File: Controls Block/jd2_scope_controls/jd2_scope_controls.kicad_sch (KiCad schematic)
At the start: 20 parts, among them SW1 RotaryEncoder_Switch, SW2 RotaryEncoder_Switch, SW3 RotaryEncoder_Switch, SW4 SW_SPST

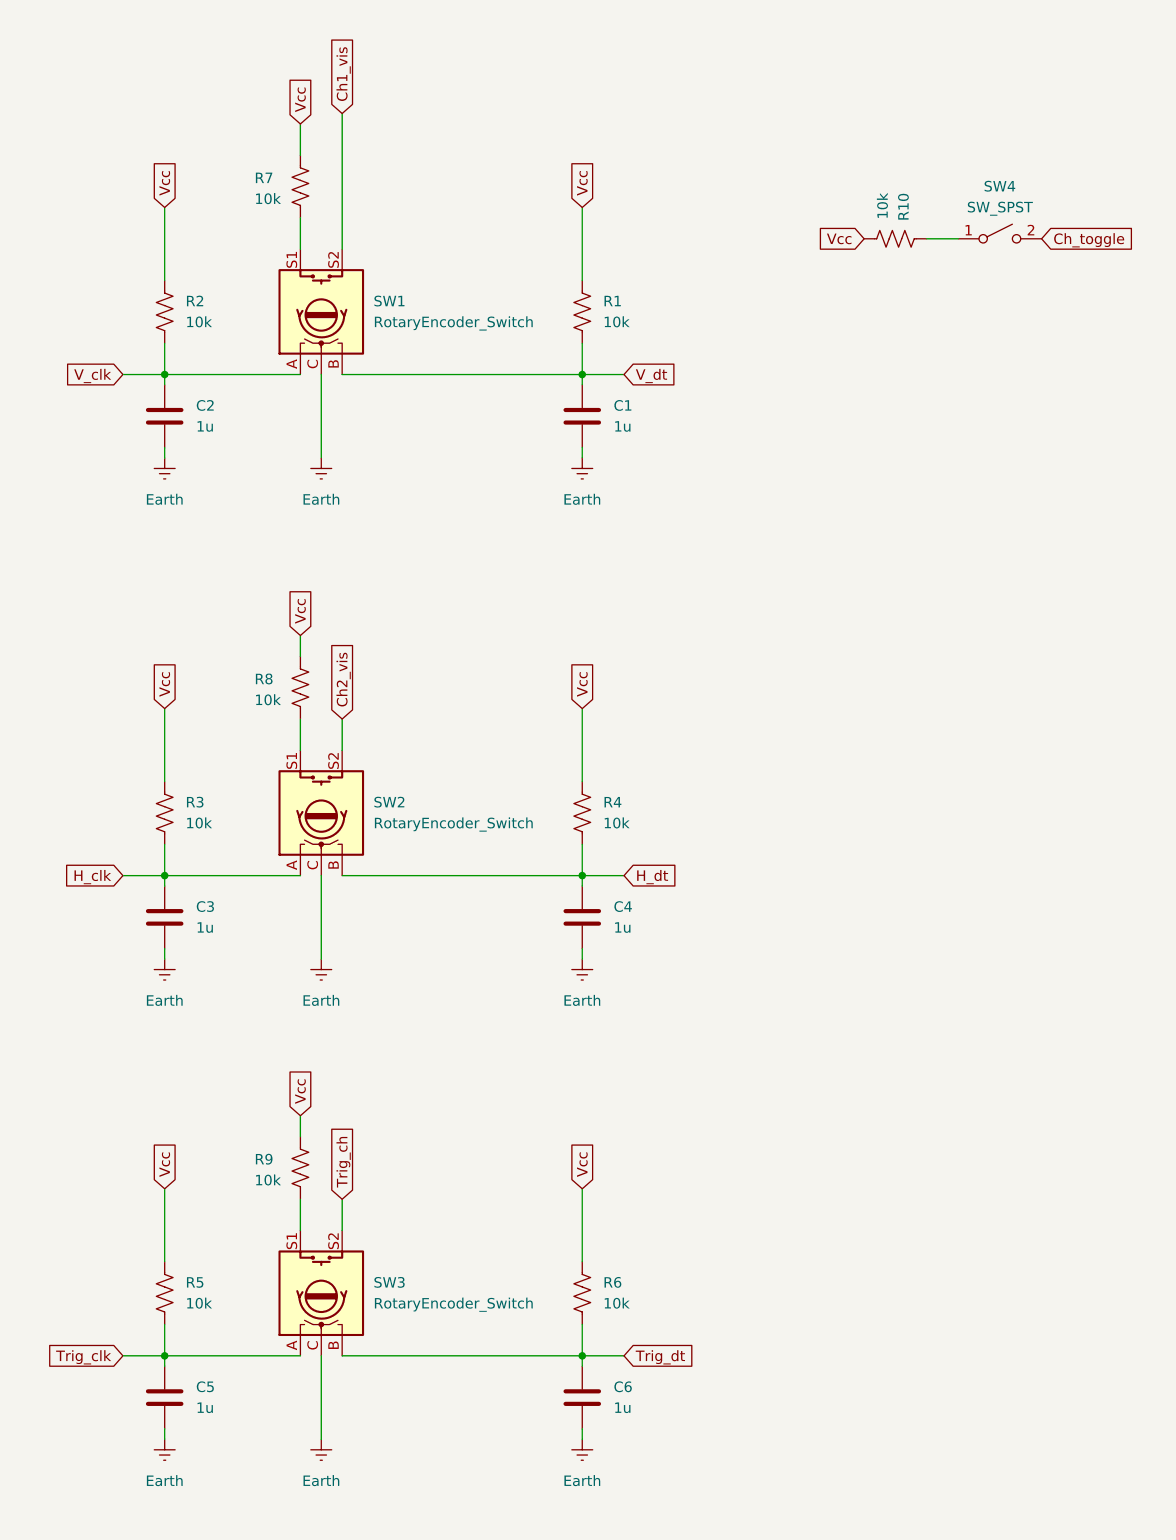
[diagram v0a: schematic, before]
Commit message: footprint stuff
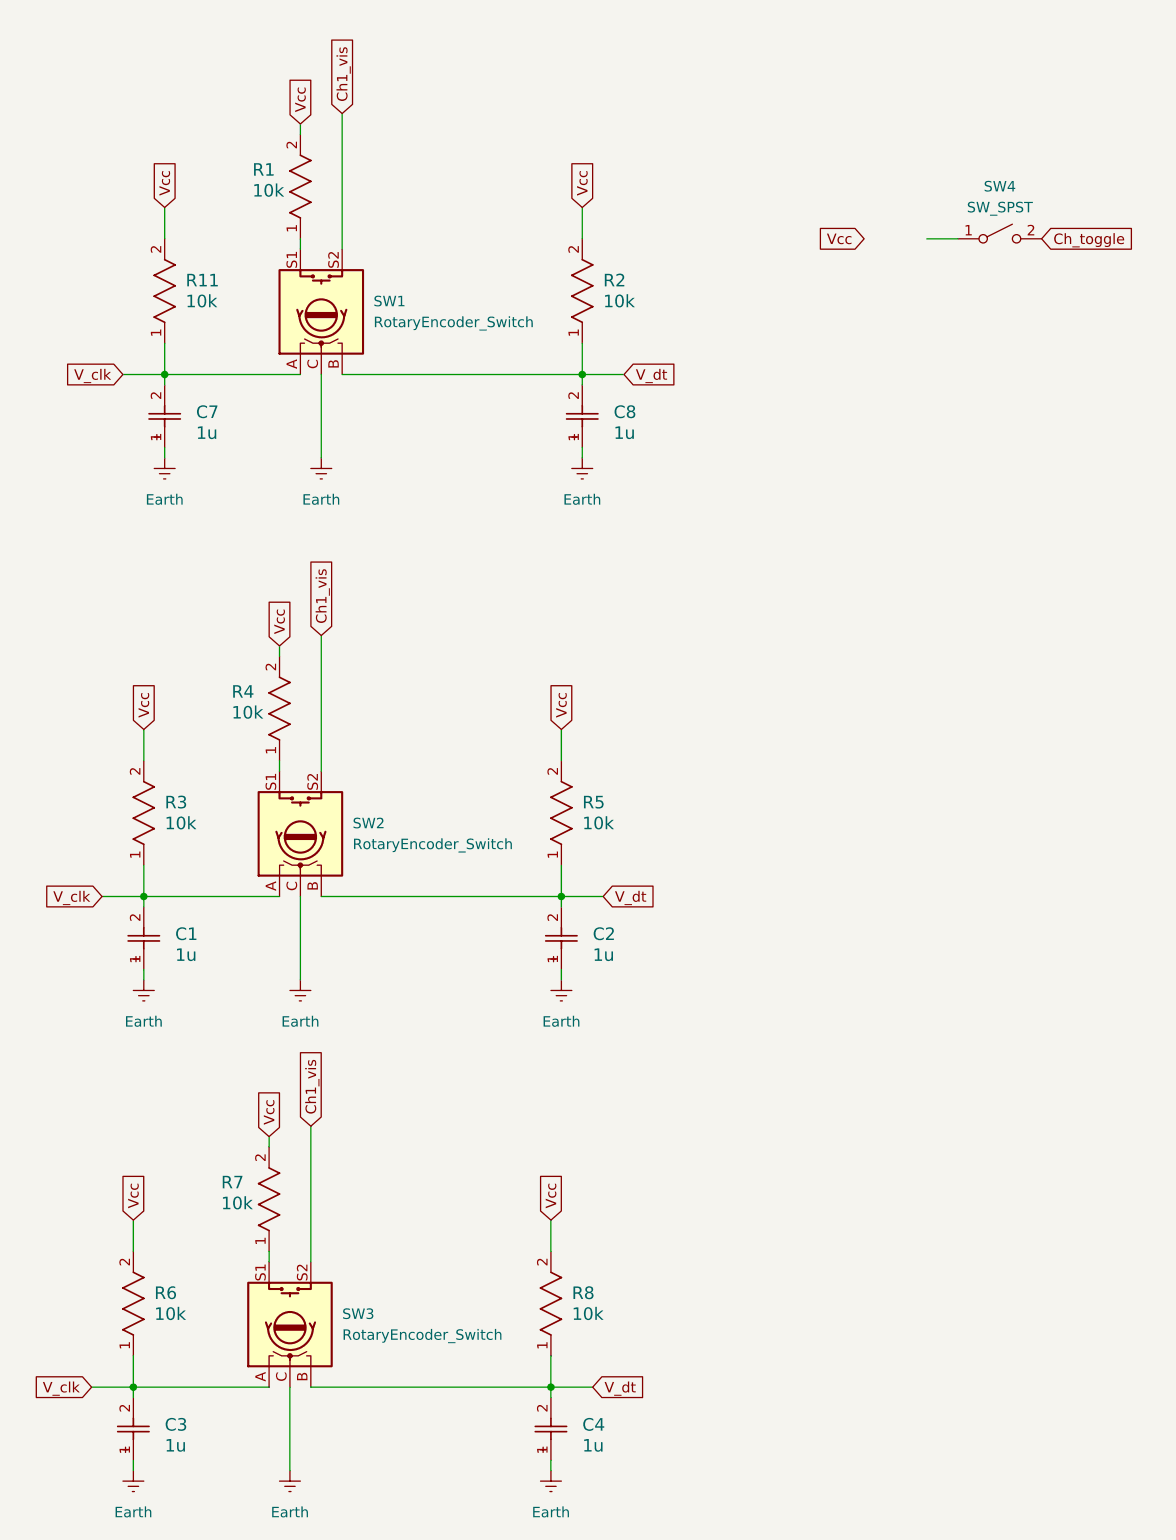
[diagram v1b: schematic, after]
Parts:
- removed C1, C2, C3, C4, C5, C6: 1u, symbol Device:C
- removed R1, R10, R2, R3, R4, R5, R6, R7, R8, R9: 10k, symbol Device:R_US
- added C1, C2, C3, C4, C7, C8: 1u, CAP_UEP_6P3X11_NCH, symbol fp1:UVZ2F010MED1TD
- added R1, R11, R2, R3, R4, R5, R6, R7, R8: 10k, STA_RMCF0402_STP, symbol fp1:RMCF0402FT10K0
- SW4: footprint (none) -> Button_Switch_SMD:Nidec_Copal_CAS-120A
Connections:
- net Ch2_vis is gone; now on net Ch1_vis: SW2.S2
- net H_clk is gone; now on net V_clk: SW2.A
- net H_dt is gone; now on net V_dt: SW2.B
- net Trig_ch is gone; now on net Ch1_vis: SW3.S2
- net Trig_clk is gone; now on net V_clk: SW3.A
- net Trig_dt is gone; now on net V_dt: SW3.B
- net Earth: now also C1.1, C2.1, C3.1, C4.1, C7.1, C8.1
- net V_clk: now also C1.2, C3.2, C7.2, R11.1, R3.1, R6.1
- net V_dt: now also C2.2, C4.2, C8.2, R2.1, R5.1, R8.1
- net Vcc: now also R1.2, R11.2, R2.2, R3.2, R4.2, R5.2, R6.2, R7.2, R8.2
- net at SW3.S1: now also R7.1
- net at SW2.S1: now also R4.1
- net at SW1.S1: now also R1.1
